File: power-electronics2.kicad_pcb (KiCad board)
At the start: 2 copper layers, 4 parts, among them J1 Vin, Q1 STP16NF06

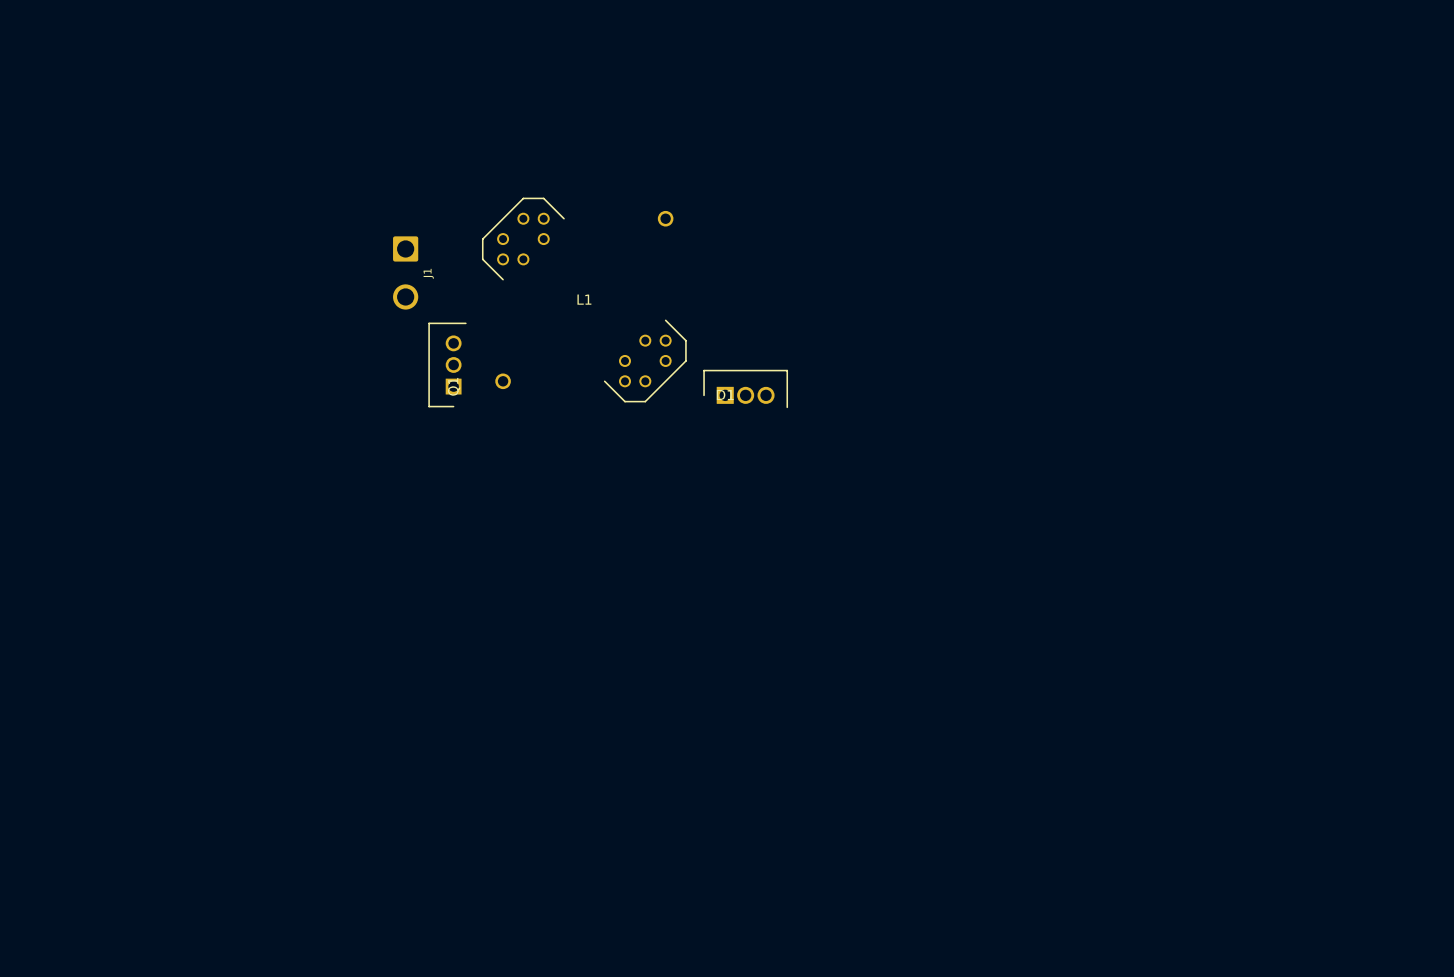
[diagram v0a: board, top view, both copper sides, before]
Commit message: add components
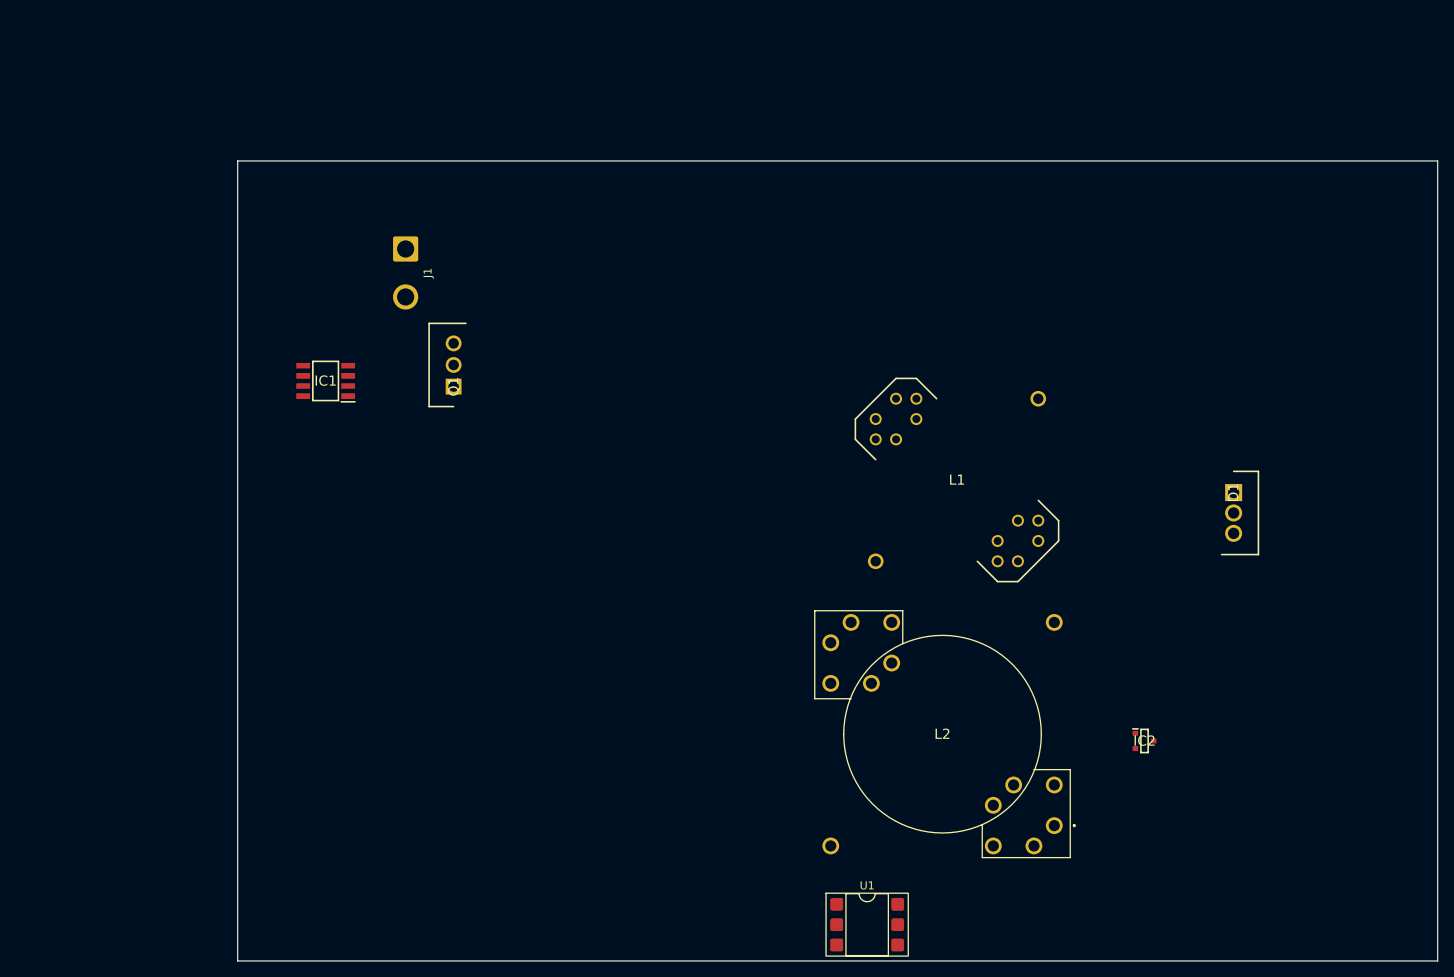
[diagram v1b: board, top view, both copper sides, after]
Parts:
- added IC1: UC2843BD1, Samacsys:SOIC127P600X175-8M, F.Cu at (59.0, 60.5)
- added IC2: ZTL431AFFTA, Samacsys:SOTFL95P240X110-3N, F.Cu at (161.4, 105.5)
- added L2: B65816N1012D001, Samacsys:B65816N1012D001, F.Cu at (150.1, 116.1)
- added U1: 4N35, Package_DIP:DIP-6_W7.62mm_SMDSocket_SmallPads, F.Cu at (126.7, 128.5)
- moved D1 64.7 mm to (172.5, 74.5), turned to -90 degrees
- moved L1 51.7 mm to (127.8, 65.3)
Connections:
- L1 pad 10: unconnected-(L1-Pad10) -> Net-(D1-A1)
- L1 pad 3: unconnected-(L1-Pad3) -> Net-(Q1-D)
- L1 pad 6: GND -> unconnected-(L1-Pad6)
- L1 pad 7: unconnected-(L1-Pad7) -> GND
- Q1 pad 1: unconnected-(Q1-G-Pad1) -> Net-(IC1-OUTPUT)
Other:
- board outline added: 150 x 100 mm

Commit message: finish pcb
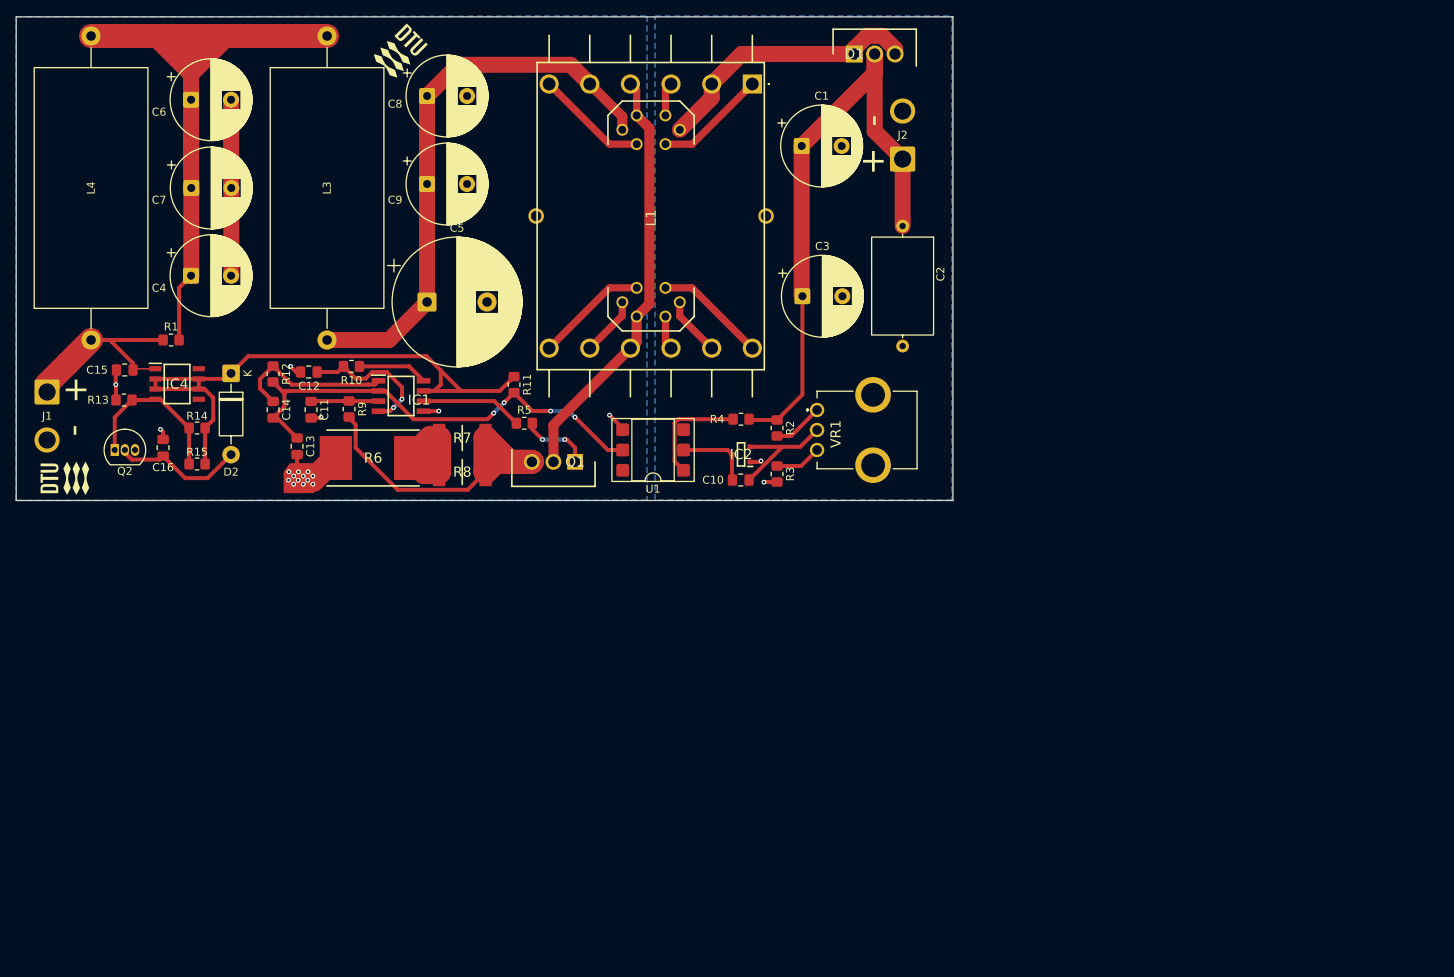
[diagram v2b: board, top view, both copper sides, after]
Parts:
- removed L2: B65816N1012D001, Samacsys:B65816N1012D001
- added C1: 47u, Capacitor_THT:CP_Radial_D10.0mm_P5.00mm, F.Cu at (118.5, 31.1)
- added C10: C, Capacitor_SMD:C_0805_2012Metric_Pad1.18x1.45mm_HandSolder, F.Cu at (110.9, 72.9)
- added C11: 1n8, Capacitor_SMD:C_0805_2012Metric_Pad1.18x1.45mm_HandSolder, F.Cu at (57.2, 64.1)
- added C12: 1n8, Capacitor_SMD:C_0805_2012Metric_Pad1.18x1.45mm_HandSolder, F.Cu at (56.9, 59.4)
- added C13: 1n6, Capacitor_SMD:C_0805_2012Metric_Pad1.18x1.45mm_HandSolder, F.Cu at (55.4, 68.7)
- added C14: 1n, Capacitor_SMD:C_0805_2012Metric_Pad1.18x1.45mm_HandSolder, F.Cu at (52.4, 64.1)
- added C15: u1, Capacitor_SMD:C_0805_2012Metric_Pad1.18x1.45mm_HandSolder, F.Cu at (33.9, 59.1)
- added C16: 22u, Capacitor_SMD:C_0805_2012Metric_Pad1.18x1.45mm_HandSolder, F.Cu at (38.7, 68.8)
- added C2: 3u3, Capacitor_THT:C_Axial_L12.0mm_D7.5mm_P15.00mm_Horizontal, F.Cu at (131.1, 41.1)
- added C3: 47u, Capacitor_THT:CP_Radial_D10.0mm_P5.00mm, F.Cu at (118.6, 49.9)
- added C4: 390u, Capacitor_THT:CP_Radial_D10.0mm_P5.00mm, F.Cu at (42.2, 47.3)
- added C5: 1170u, Capacitor_THT:CP_Radial_D16.0mm_P7.50mm, F.Cu at (71.7, 50.6)
- added C6: C, Capacitor_THT:CP_Radial_D10.0mm_P5.00mm, F.Cu at (42.2, 25.3)
- added C7: C, Capacitor_THT:CP_Radial_D10.0mm_P5.00mm, F.Cu at (42.2, 36.4)
- added C8: C, Capacitor_THT:CP_Radial_D10.0mm_P5.00mm, F.Cu at (71.7, 24.9)
- added C9: C, Capacitor_THT:CP_Radial_D10.0mm_P5.00mm, F.Cu at (71.7, 35.9)
- added D2: 1N4005, Diode_THT:D_DO-41_SOD81_P10.16mm_Horizontal, F.Cu at (47.2, 59.5)
- added G***: LOGO, Samacsys:dtulogo, F.Cu at (68.3, 19.3)
- added G***: LOGO, Samacsys:dtulogo, F.Cu at (26.4, 72.6)
- added H1: B65816C1512T001, Samacsys:B65816C1512T001, F.Cu at (112.3, 23.4)
- added IC4: LM317LD, Samacsys:SOIC127P600X175-8N, F.Cu at (40.4, 60.9)
- added J2: Vo, Connector_Wire:SolderWire-1.5sqmm_1x02_P6mm_D1.7mm_OD3mm, F.Cu at (131.1, 32.8)
- added L3: 123u, Inductor_THT:L_Axial_L29.9mm_D14.0mm_P38.00mm_Horizontal_Vishay_IHA-105, F.Cu at (59.2, 17.4)
- added L4: 470u, Inductor_THT:L_Axial_L29.9mm_D14.0mm_P38.00mm_Horizontal_Vishay_IHA-105, F.Cu at (29.7, 55.4)
- added Q2: 2N3906, Package_TO_SOT_THT:TO-92_Inline, F.Cu at (32.6, 69.1)
- added R1: 445m, Resistor_SMD:R_0805_2012Metric_Pad1.20x1.40mm_HandSolder, F.Cu at (39.7, 55.4)
- added R10: 10k, Resistor_SMD:R_0805_2012Metric_Pad1.20x1.40mm_HandSolder, F.Cu at (62.2, 58.7)
- added R11: 12k3, Resistor_SMD:R_0805_2012Metric_Pad1.20x1.40mm_HandSolder, F.Cu at (82.5, 61.0)
- added R12: 10k, Resistor_SMD:R_0805_2012Metric_Pad1.20x1.40mm_HandSolder, F.Cu at (52.4, 59.6)
- added R13: 2k7, Resistor_SMD:R_0805_2012Metric_Pad1.20x1.40mm_HandSolder, F.Cu at (33.8, 62.9)
- added R14: 240R, Resistor_SMD:R_0805_2012Metric_Pad1.20x1.40mm_HandSolder, F.Cu at (42.9, 66.4)
- added R15: 50k, Resistor_SMD:R_0805_2012Metric_Pad1.20x1.40mm_HandSolder, F.Cu at (42.9, 70.9)
- added R2: R, Resistor_SMD:R_0805_2012Metric_Pad1.20x1.40mm_HandSolder, F.Cu at (115.4, 66.4)
- added R3: R, Resistor_SMD:R_0805_2012Metric_Pad1.20x1.40mm_HandSolder, F.Cu at (115.4, 72.1)
- added R4: R, Resistor_SMD:R_0805_2012Metric_Pad1.20x1.40mm_HandSolder, F.Cu at (110.9, 65.3)
- added R5: 10R, Resistor_SMD:R_0805_2012Metric_Pad1.20x1.40mm_HandSolder, F.Cu at (83.8, 65.8)
- added R6: WSR5R1000FEA, Samacsys:RESM11670X254N, F.Cu at (64.9, 70.1)
- added R7: CRA2512-FZ-R050ELF, Samacsys:RESC6434X90N, F.Cu at (76.1, 67.6)
- added R8: CRA2512-FZ-R050ELF, Samacsys:RESC6434X90N, F.Cu at (76.1, 71.9)
- added R9: 100R, Resistor_SMD:R_0805_2012Metric_Pad1.20x1.40mm_HandSolder, F.Cu at (61.9, 64.0)
- added VR1: PTV09A-4020F-B104, Samacsys:PTV09A4020FB103, F.Cu at (126.0, 66.6)
- moved D1 72.5 mm to (125.1, 19.6), turned to 0 degrees
- moved U1 65.1 mm to (99.9, 69.1), turned to 180 degrees
- moved IC2 61.9 mm to (110.9, 69.7), turned to 180 degrees
- moved L1 48.3 mm to (97.9, 27.3), turned to -45 degrees
- moved J1 48.3 mm to (24.2, 61.9)
- moved Q1 17.9 mm to (90.2, 70.6), turned to 180 degrees
- moved IC1 9.61 mm to (68.4, 62.4), turned to 0 degrees
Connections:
- D1 pad 1: Net-(D1-A1) -> /Vs+
- D1 pad 2: unconnected-(D1-K-Pad2) -> /Vo
- D1 pad 3: Net-(D1-A1) -> /Vs+
- IC1 pad 1: unconnected-(IC1-COMP-Pad1) -> Net-(IC1-COMP)
- IC1 pad 2: unconnected-(IC1-VFB-Pad2) -> Net-(IC1-VFB)
- IC1 pad 3: unconnected-(IC1-ISENSE-Pad3) -> Net-(IC1-ISENSE)
- IC1 pad 4: unconnected-(IC1-RT/CT-Pad4) -> Net-(IC1-RT/CT)
- IC1 pad 7: unconnected-(IC1-VI-Pad7) -> /Vldo
- IC1 pad 8: unconnected-(IC1-VREF-Pad8) -> Net-(IC1-VREF)
- IC2 pad 1: unconnected-(IC2-ANODE-Pad1) -> GND
- IC2 pad 2: unconnected-(IC2-REF-Pad2) -> Net-(IC2-REF)
- IC2 pad 3: unconnected-(IC2-CATHODE-Pad3) -> Net-(IC2-CATHODE)
- J1 pad 1: Net-(J1-Pin_1) -> /Vi
- L1 pad 1: Net-(J1-Pin_1) -> /Vp-
- L1 pad 10: Net-(D1-A1) -> Net-(H1-Pad1)
- L1 pad 11: unconnected-(L1-Pad11) -> /Vs+
- L1 pad 12: unconnected-(L1-Pad12) -> GND
- L1 pad 2: unconnected-(L1-Pad2) -> /Vp+
- L1 pad 3: Net-(Q1-D) -> Net-(H1-Pad6)
- L1 pad 4: Net-(Q1-D) -> Net-(H1-Pad7)
- L1 pad 5: unconnected-(L1-Pad5) -> Net-(H1-Pad8)
- L1 pad 6: unconnected-(L1-Pad6) -> /Vp-
- L1 pad 8: unconnected-(L1-Pad8) -> Net-(H1-Pad11)
- L1 pad 9: Net-(D1-A1) -> Net-(H1-Pad12)
- Q1 pad 1: Net-(IC1-OUTPUT) -> Net-(Q1-G)
- Q1 pad 2: Net-(Q1-D) -> /Vp-
- Q1 pad 3: GNDREF -> Net-(Q1-S)
- U1 pad 1: unconnected-(U1-Pad1) -> Net-(R4-Pad2)
- U1 pad 2: unconnected-(U1-Pad2) -> Net-(IC2-CATHODE)
- U1 pad 4: unconnected-(U1-Pad4) -> GNDREF
- U1 pad 5: unconnected-(U1-Pad5) -> Net-(IC1-VFB)
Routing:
- net /Vo: track 0.00 -> 77.4 mm
- net /Vldo: track 0.00 -> 77.4 mm
- net Net-(C4-Pad1): track 0.00 -> 77.0 mm
- net /Vp+: track 0.00 -> 70.6 mm
- net Net-(IC1-VFB): track 0.00 -> 59.6 mm, vias 0 -> 4
- net /Vp-: track 0.00 -> 53.2 mm
- net GNDREF: track 0.00 -> 42.7 mm, vias 0 -> 18
- net Net-(Q1-S): track 0.00 -> 41.0 mm
- net /Vs+: track 0.00 -> 34.5 mm
- net /Vi: track 0.00 -> 27.9 mm
- net Net-(IC4-ADJ): track 0.00 -> 20.3 mm
- net Net-(IC1-COMP): track 0.00 -> 20.1 mm
- net Net-(IC1-RT/CT): track 0.00 -> 17.7 mm, vias 0 -> 2
- net Net-(D2-A): track 0.00 -> 16.5 mm
- net Net-(IC2-REF): track 0.00 -> 15.1 mm
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- added copper zone on B.Cu, net GND
- added copper zone on B.Cu, net GNDREF
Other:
- board size 150 x 100 mm -> 117.1 x 60.5 mm
